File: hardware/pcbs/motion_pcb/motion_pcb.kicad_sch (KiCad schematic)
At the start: 23 parts, among them J1 esp_io_shield1, J2 esp_io_shield2, J3 esp32_voltage_shield, J4 Con_top_pcb, J5 con_rpi, SW1 SW_Push, U4 74HC4051

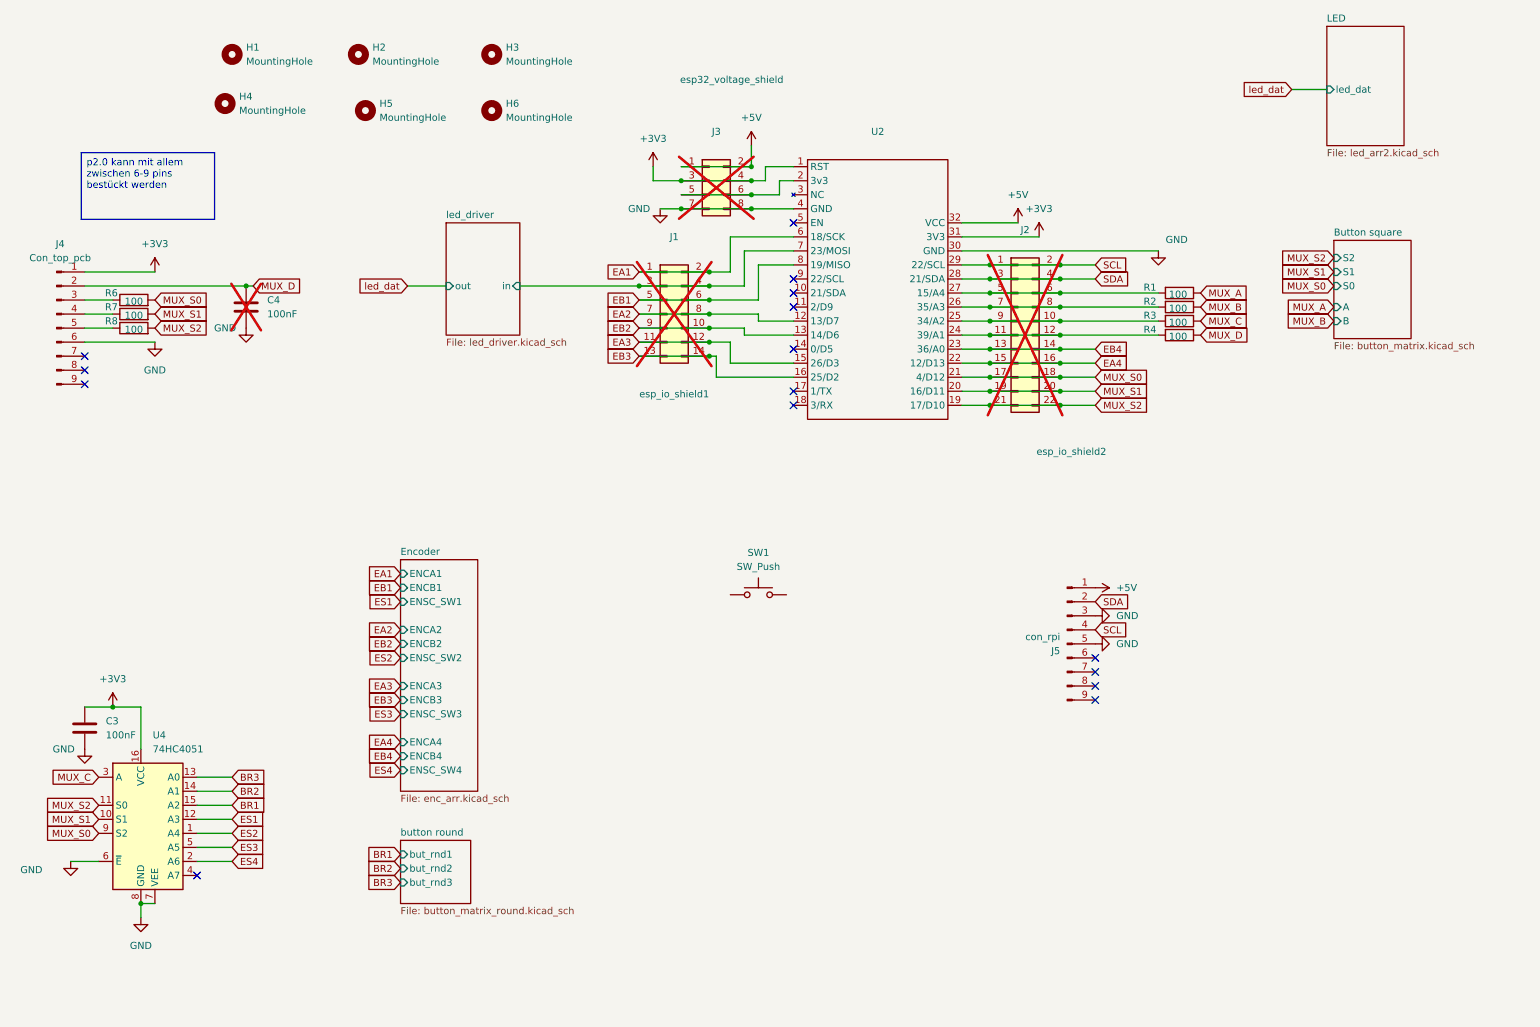
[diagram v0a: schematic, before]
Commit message: finished schematic
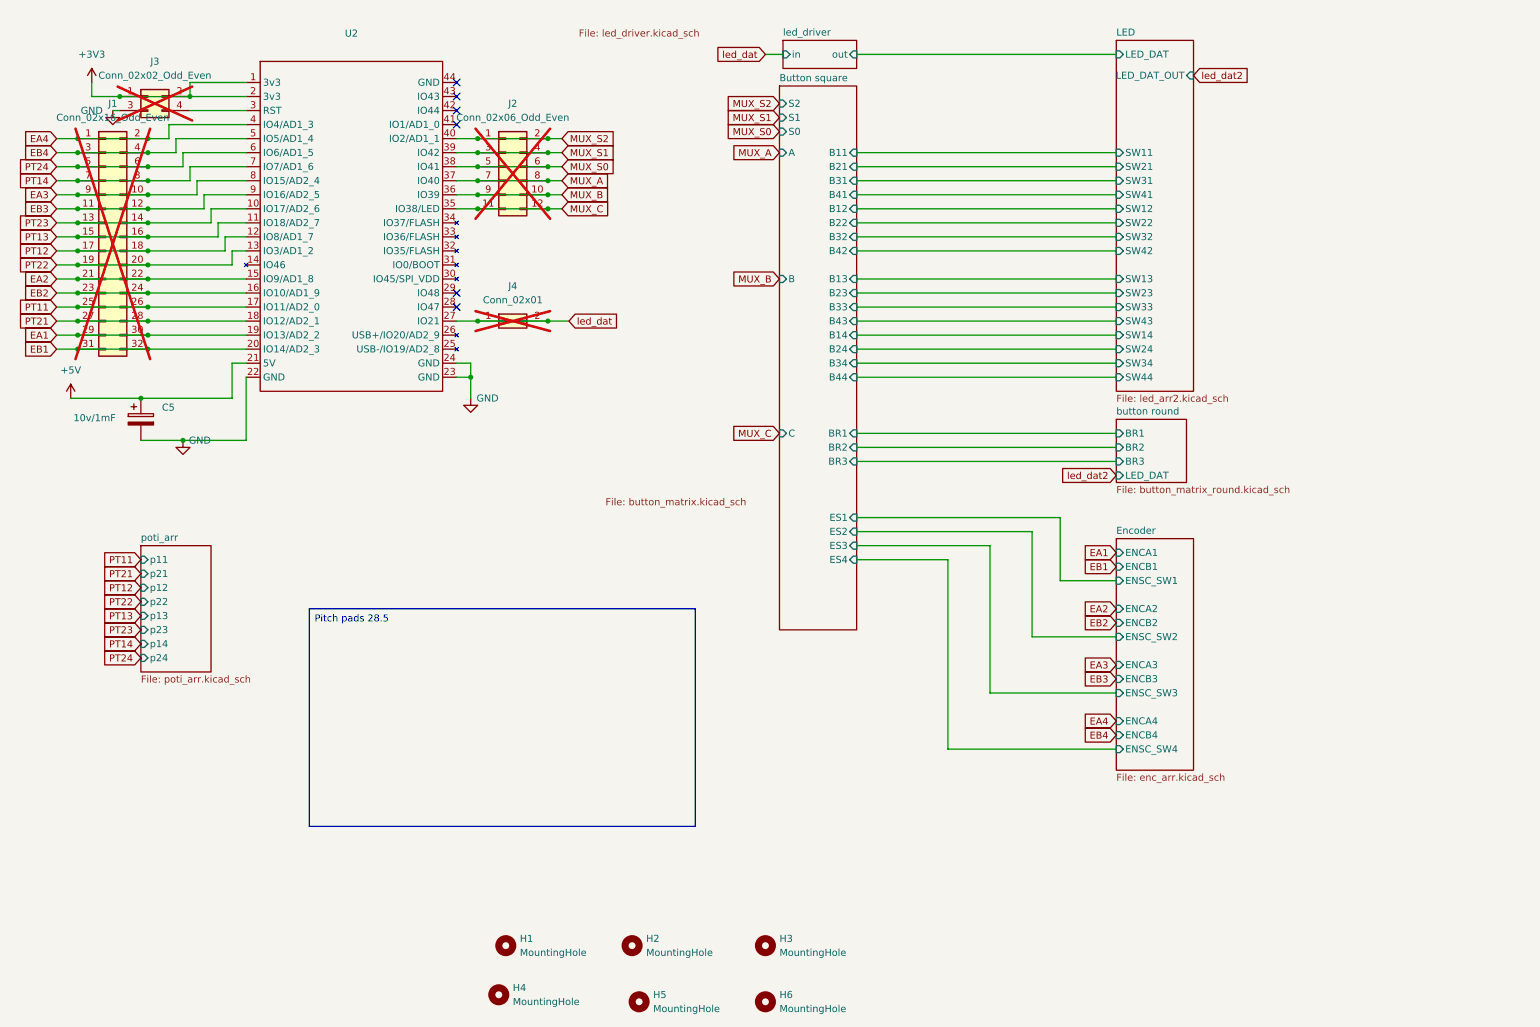
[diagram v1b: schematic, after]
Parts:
- removed C3, C4: 100nF, Capacitor_SMD:C_1206_3216Metric_Pad1.33x1.80mm_HandSolder, symbol Device:C
- removed J1: esp_io_shield1, Connector_PinHeader_2.54mm:PinHeader_2x07_P2.54mm_Vertical_SMD, symbol Connector_Generic:Conn_02x07_Odd_Even
- removed J2: esp_io_shield2, Connector_PinHeader_2.54mm:PinHeader_2x11_P2.54mm_Vertical_SMD, symbol Connector_Generic:Conn_02x11_Odd_Even
- removed J3: esp32_voltage_shield, Connector_PinHeader_2.54mm:PinHeader_2x04_P2.54mm_Vertical_SMD, symbol Connector_Generic:Conn_02x04_Odd_Even
- removed J4: Con_top_pcb, Connector_JST:JST_PH_B9B-PH-K_1x09_P2.00mm_Vertical, symbol Connector:Conn_01x09_Pin
- removed J5: con_rpi, Connector_JST:JST_PH_B9B-PH-K_1x09_P2.00mm_Vertical, symbol Connector:Conn_01x09_Pin
- removed R1, R2, R3, R4, R6, R7, R8: 100, Resistor_SMD:R_1206_3216Metric_Pad1.30x1.75mm_HandSolder, symbol Device:R
- removed SW1: SW_Push, symbol Switch:SW_Push
- removed U2: ~, esp32:DFR0645, symbol esp32:DFR0654
- removed U4: 74HC4051, Package_SO:SOIC-16_3.9x9.9mm_P1.27mm, symbol 74xx:74HC4051
- added C5: 10v/1mF, Capacitor_SMD:CP_Elec_10x10, symbol Device:C_Polarized
- added J1: Conn_02x16_Odd_Even, symbol Connector_Generic:Conn_02x16_Odd_Even
- added J2: Conn_02x06_Odd_Even, symbol Connector_Generic:Conn_02x06_Odd_Even
- added J3: Conn_02x02_Odd_Even, symbol Connector_Generic:Conn_02x02_Odd_Even
- added J4: Conn_02x01, symbol Connector_Generic:Conn_02x01
- added U2: ~, 3dAudioFoot:ESP32-S3-DevKitC-1, symbol 3dAudioSym:ESP32_S3_DevKit_C1
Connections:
- net +3V3: now also J3.1 (Pin_1), J3.2 (Pin_2), U2.1 (3v3), U2.2 (3v3)
- net +5V: now also C5.1, U2.21 (5V)
- net EA1: now also J1.29 (Pin_29), J1.30 (Pin_30), U2.19 (IO13/AD2_2)
- net EA2: now also J1.21 (Pin_21), J1.22 (Pin_22), U2.15 (IO9/AD1_8)
- net EA3: now also J1.10 (Pin_10), J1.9 (Pin_9), U2.8 (IO15/AD2_4)
- net EA4: now also J1.1 (Pin_1), J1.2 (Pin_2), U2.4 (IO4/AD1_3)
- net EB1: now also J1.31 (Pin_31), J1.32 (Pin_32), U2.20 (IO14/AD2_3)
- net EB2: now also J1.23 (Pin_23), J1.24 (Pin_24), U2.16 (IO10/AD1_9)
- net EB3: now also J1.11 (Pin_11), J1.12 (Pin_12), U2.9 (IO16/AD2_5)
- net EB4: now also J1.3 (Pin_3), J1.4 (Pin_4), U2.5 (IO5/AD1_4)
- net GND: now also C5.2, J3.3 (Pin_3), U2.22 (GND), U2.23 (GND), U2.24 (GND)
- net MUX_A: now also J2.7 (Pin_7), J2.8 (Pin_8), U2.37 (IO40)
- net MUX_B: now also J2.10 (Pin_10), J2.9 (Pin_9), U2.36 (IO39)
- net MUX_C: now also J2.11 (Pin_11), J2.12 (Pin_12), U2.35 (IO38/LED)
- net MUX_S0: now also J2.5 (Pin_5), J2.6 (Pin_6), U2.38 (IO41)
- net MUX_S1: now also J2.3 (Pin_3), J2.4 (Pin_4), U2.39 (IO42)
- net MUX_S2: now also J2.1 (Pin_1), J2.2 (Pin_2), U2.40 (IO2/AD1_1)
- net led_dat: now also J4.1 (Pin_1), J4.2 (Pin_2), U2.27 (IO21)
- new net: J3.4 (Pin_4), U2.3 (RST)
- new net PT11: J1.25 (Pin_25), J1.26 (Pin_26), U2.17 (IO11/AD2_0)
- new net PT12: J1.17 (Pin_17), J1.18 (Pin_18), U2.12 (IO8/AD1_7)
- new net PT13: J1.15 (Pin_15), J1.16 (Pin_16), U2.11 (IO18/AD2_7)
- new net PT14: J1.7 (Pin_7), J1.8 (Pin_8), U2.7 (IO7/AD1_6)
- new net PT21: J1.27 (Pin_27), J1.28 (Pin_28), U2.18 (IO12/AD2_1)
- new net PT22: J1.19 (Pin_19), J1.20 (Pin_20), U2.13 (IO3/AD1_2)
- new net PT23: J1.13 (Pin_13), J1.14 (Pin_14), U2.10 (IO17/AD2_6)
- new net PT24: J1.5 (Pin_5), J1.6 (Pin_6), U2.6 (IO6/AD1_5)
- no-connect marks 15 -> 6
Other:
- added sheet poti_arr (poti_arr.kicad_sch)
- sheet Button square ports: added B11, B12, B13, B14, B21, B22, B23, B24, B31, B32, B33, B34, B41, B42, B43, B44, BR1, BR2, BR3, C, ES1, ES2, ES3, ES4; removed none
- sheet LED ports: added LED_DAT, LED_DAT_OUT, SW11, SW12, SW13, SW14, SW21, SW22, SW23, SW24, SW31, SW32, SW33, SW34, SW41, SW42, SW43, SW44; removed led_dat
- sheet button round ports: added BR1, BR2, BR3, LED_DAT; removed but_rnd1, but_rnd2, but_rnd3
- moved on the sheet: H1, H2, H3, H4, H5, H6
